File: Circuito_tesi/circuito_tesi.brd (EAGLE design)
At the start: 100 x 80 mm, 35 parts, among them IC3.3 317T, IC5 317T, U1 NRF52832, U2 BME688, U3 MICS-6814, U4 OPA2277PA, U5 OPA2277PA

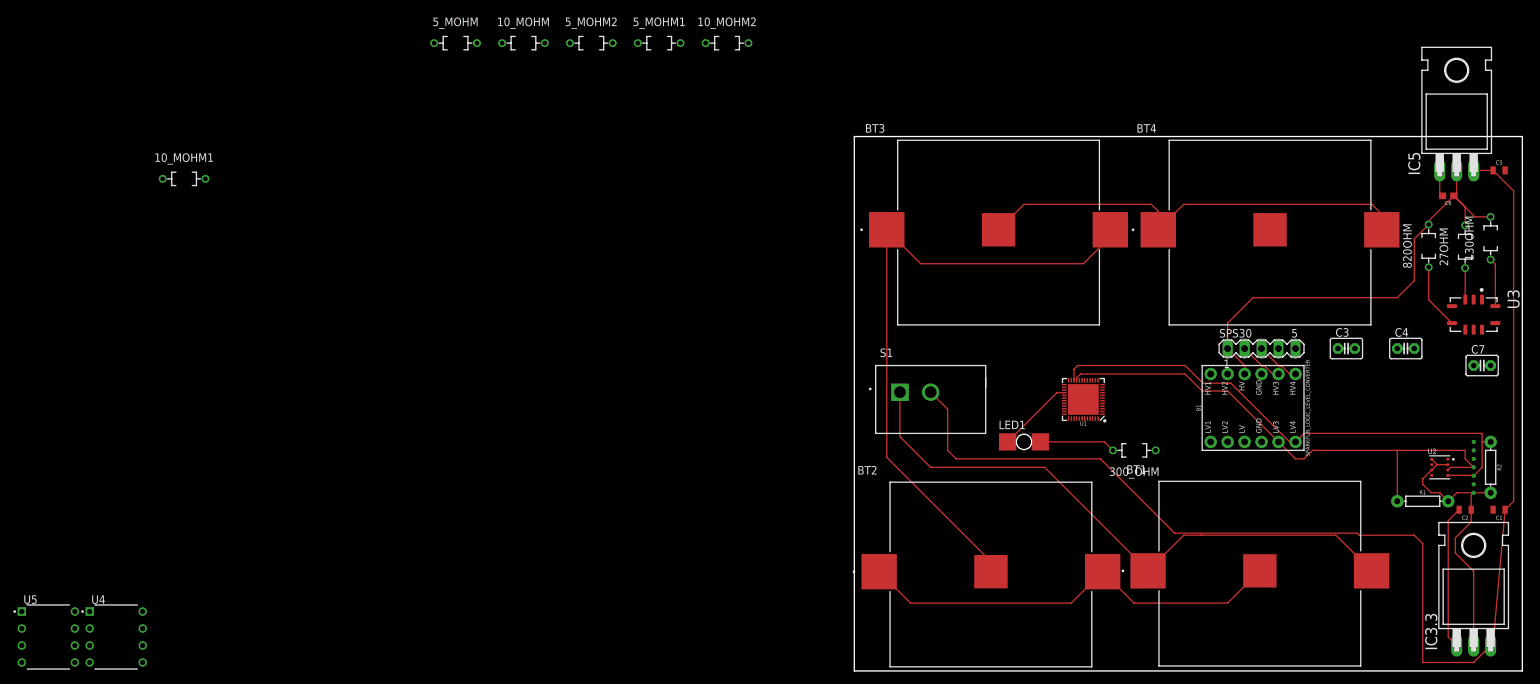
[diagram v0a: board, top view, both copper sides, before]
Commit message: Aggiunti circuiti su board
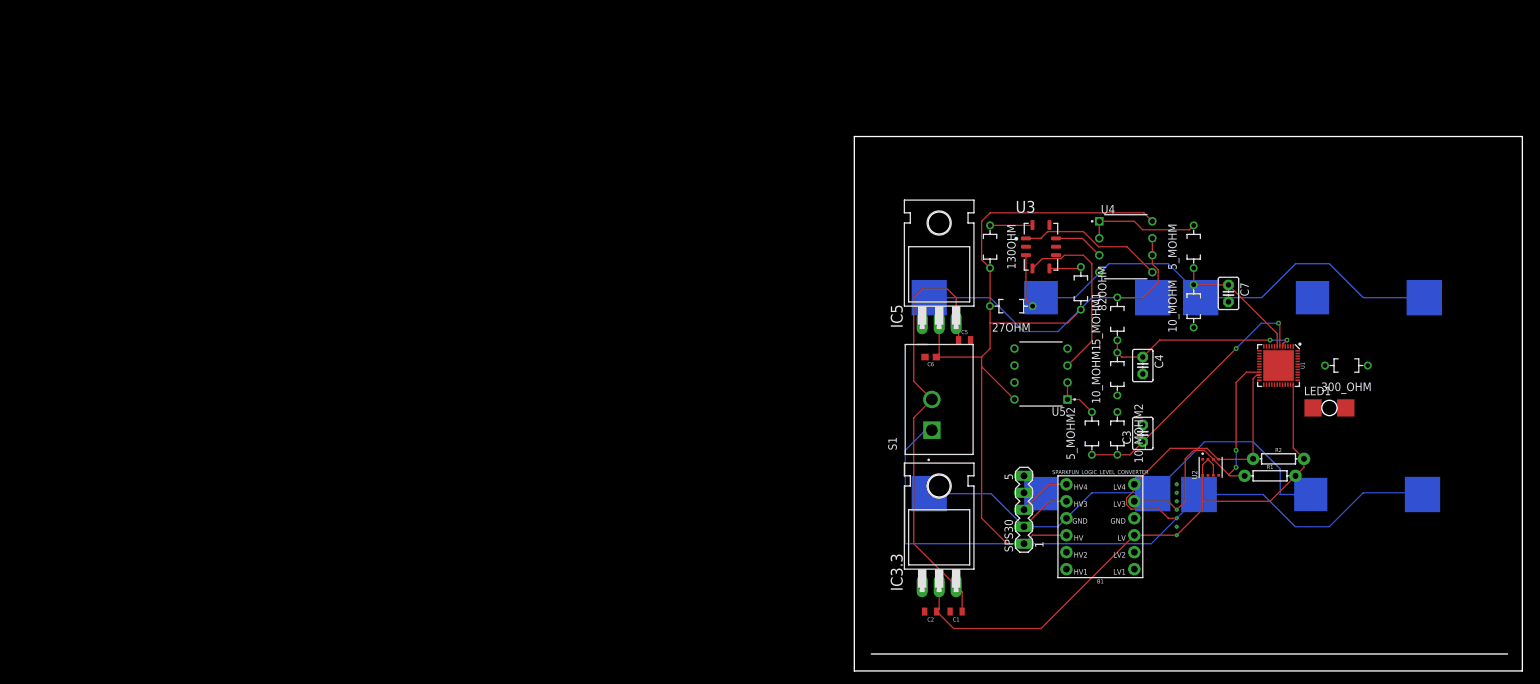
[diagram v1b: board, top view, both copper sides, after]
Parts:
- moved U4 162.0 mm to (40.6, 63.5)
- moved U5 153.7 mm to (27.9, 44.5), turned to 180 degrees
- moved 10_MOHM1 142.7 mm to (39.4, 44.5), turned to 90 degrees
- moved 5_MOHM 114.6 mm to (50.8, 63.5), turned to 90 degrees
- moved 10_MOHM 107.8 mm to (50.8, 54.6), turned to 90 degrees
- moved 5_MOHM2 95.0 mm to (35.6, 35.6), turned to 90 degrees
- moved C5 83.9 mm to (16.5, 49.5)
- moved C1 82.7 mm to (15.2, 8.89)
- moved 10_MOHM2 82.6 mm to (39.4, 35.6), turned to 270 degrees
- moved C2 81.4 mm to (11.4, 8.89)
- moved C6 81.1 mm to (11.4, 47.0)
- moved IC5 80.8 mm to (12.7, 62.2)
- moved IC3.3 80.5 mm to (12.7, 22.9)
- moved 5_MOHM1 80.0 mm to (39.4, 52.7), turned to 90 degrees
- moved 130OHM 74.9 mm to (20.3, 63.5), turned to 270 degrees
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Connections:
- net 3.3: no longer B1.GND1, B1.GND2
- net GND: now also B1.GND1, B1.GND2
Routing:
- net VDD: track 191.7 -> 66.2 mm
- net N$4: track 95.9 -> 37.7 mm
- net 5V: track 70.3 -> 120.3 mm
- net 3.3: track 43.4 -> 93.1 mm
- net N$16: track 0.00 -> 39.7 mm, vias 0 -> 2
- net SDA: track 79.3 -> 44.4 mm, vias 0 -> 2
- net SCL: track 80.3 -> 45.8 mm
- net N$18: track 0.00 -> 29.9 mm, vias 0 -> 2
- net N$14: track 0.00 -> 27.0 mm
- net GND: track 25.5 -> 0.00 mm
- net N$6: track 0.00 -> 21.9 mm
- net N$17: track 0.00 -> 19.9 mm
- net N$22: track 0.00 -> 17.5 mm
- net N$19: track 90.0 -> 104.0 mm
- net N$7: track 0.00 -> 14.0 mm
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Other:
- outline, holes or cut-outs redrawn
